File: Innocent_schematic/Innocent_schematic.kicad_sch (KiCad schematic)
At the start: 37 parts, among them IC1 MP2338GTL-Z, P1 USB_C_Plug_USB2.0, U1 CH224K, U2 TP4056-42-ESOP8, U3 MP3423GG-Z, U4 RT6150AGQW, U5 INA219AxD

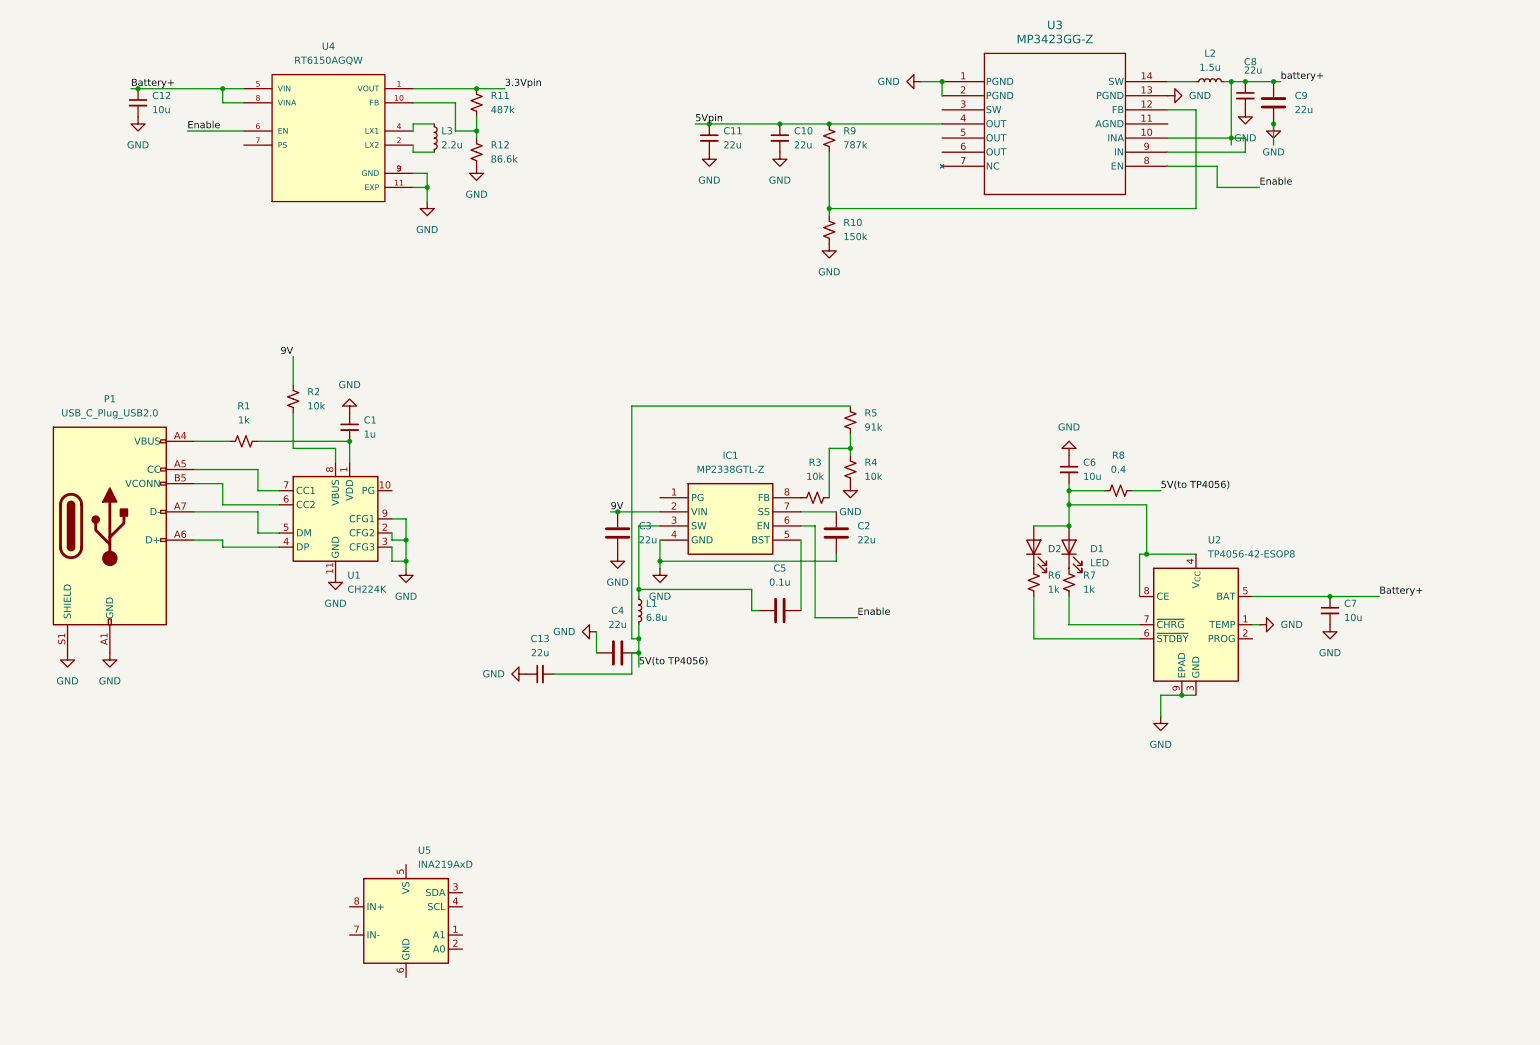
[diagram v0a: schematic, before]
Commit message: i have integrated all the systems into one project
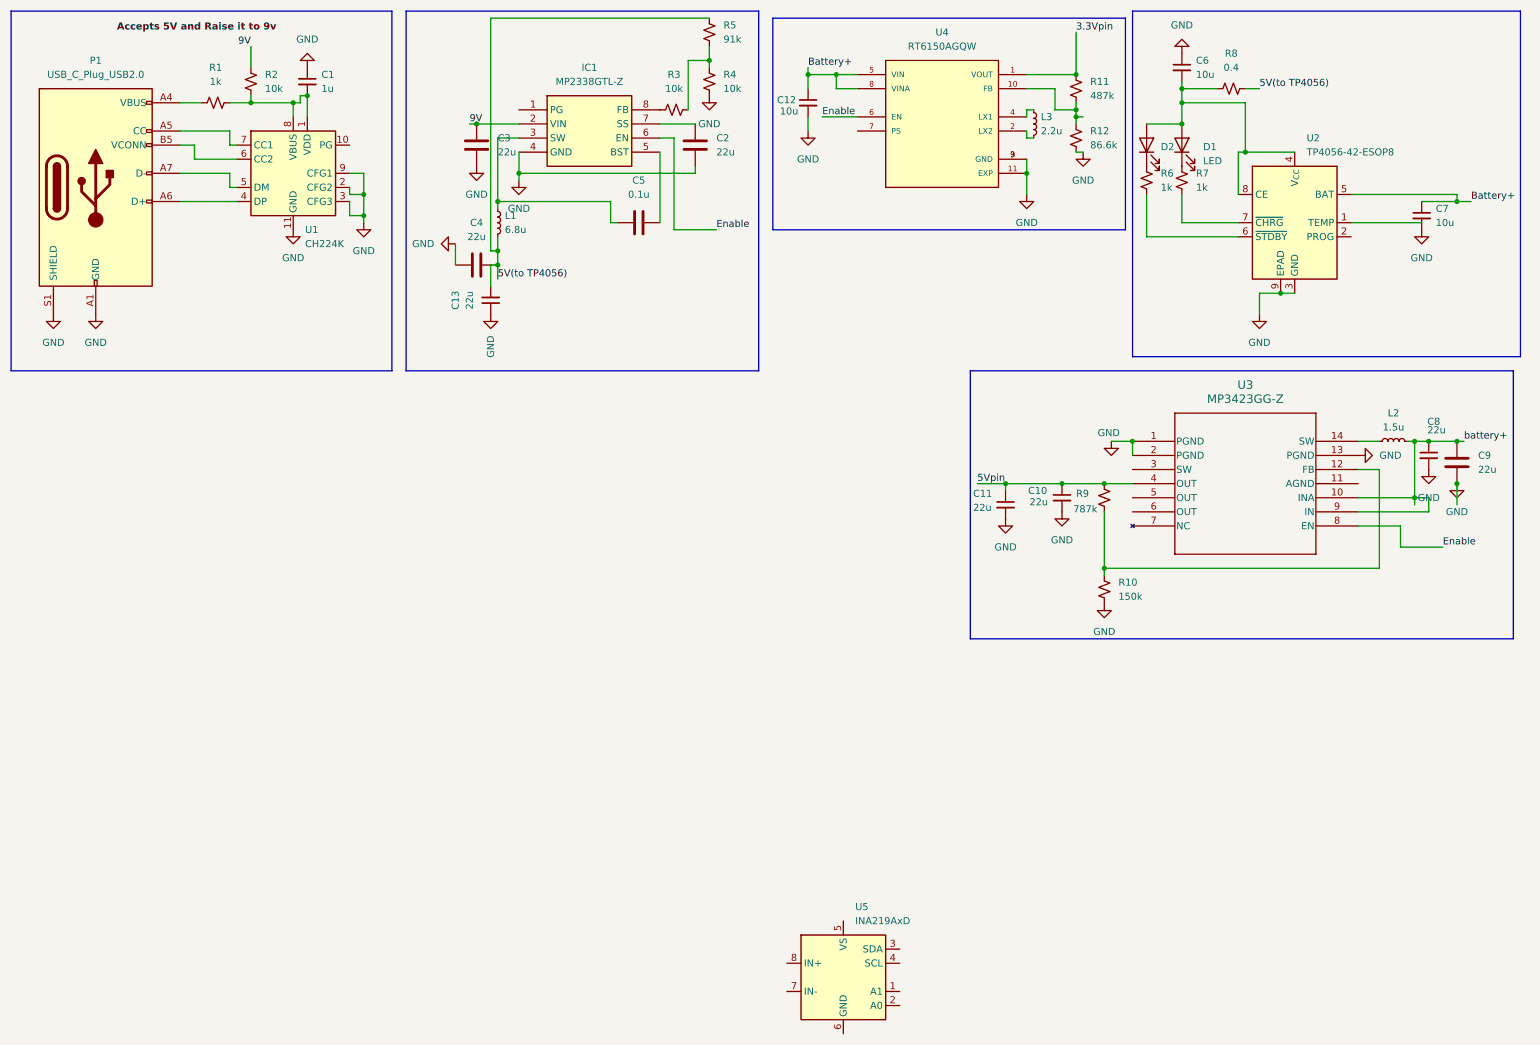
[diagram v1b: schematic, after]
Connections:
- net GND: no longer U2.1 (TEMP)
- net at C1.2, R1.2, U1.1 (VDD): now also R2.2, U1.8 (VBUS)
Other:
- moved on the sheet: C1, C10, C11, C12, C13, C2, C3, C4, C5, C6, C7, C8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
